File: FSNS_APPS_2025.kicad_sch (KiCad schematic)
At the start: 28 parts, among them J1 Conn_01x04_Pin, J2 Conn_01x03_Pin, J3 Conn_01x03_Pin, U1 STM32F103C8T6, U2 MCP6001-OT, U3 MCP6001-OT, Y1 16MHz

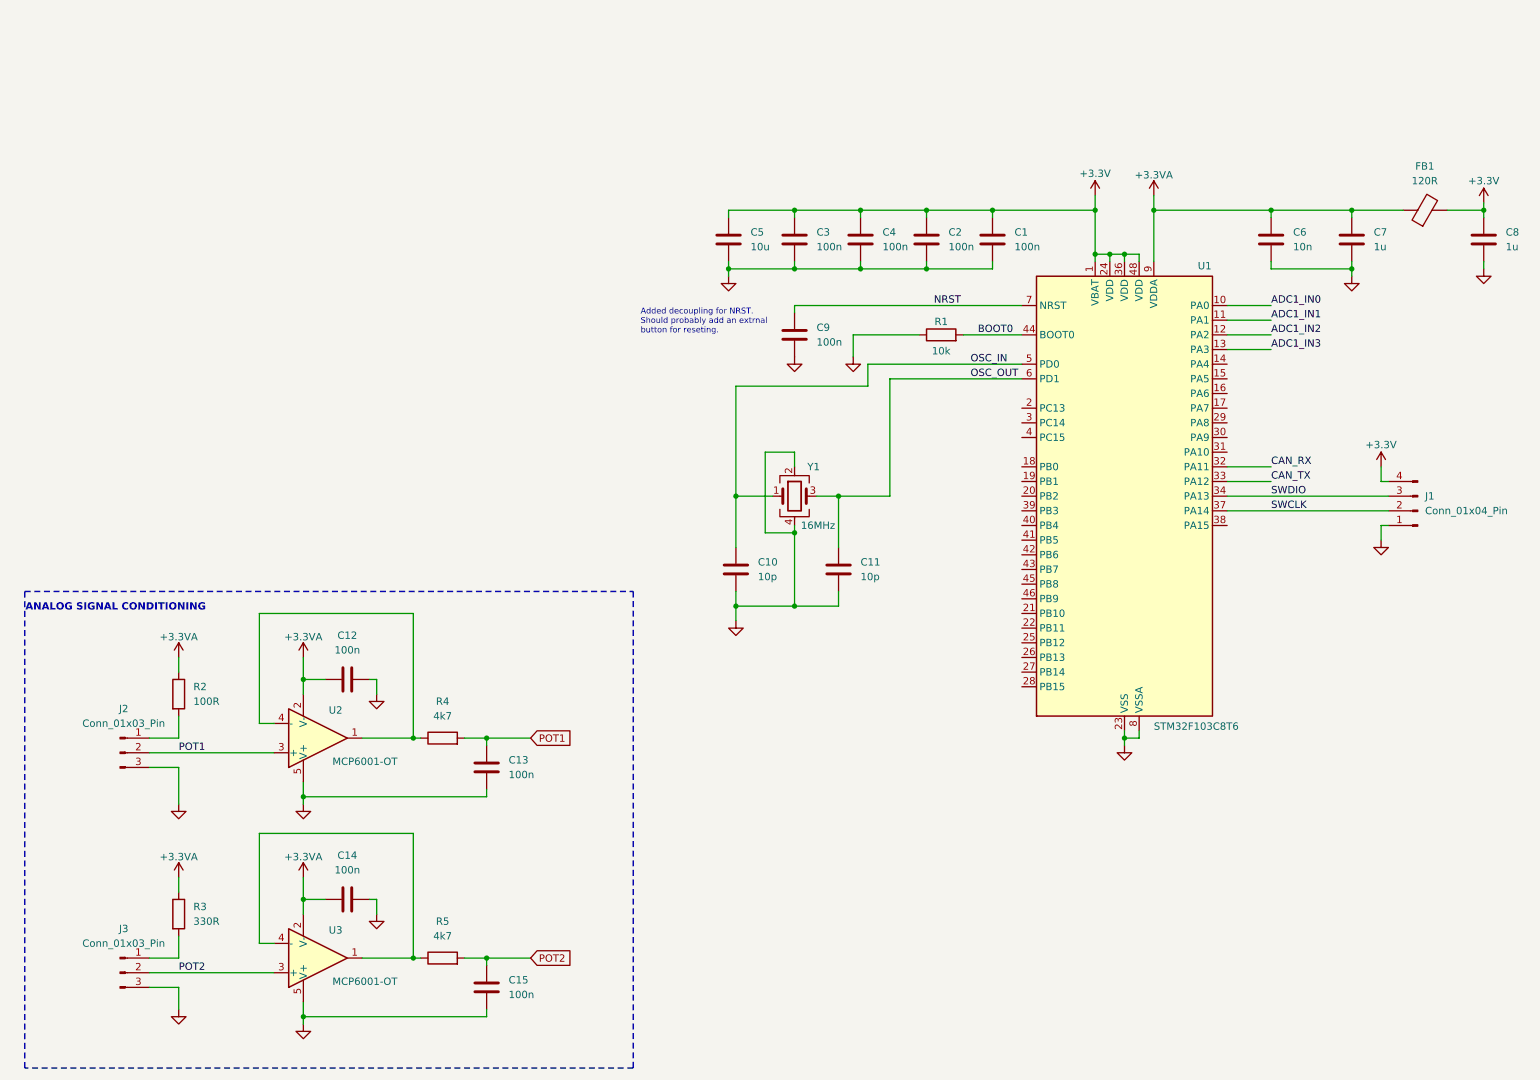
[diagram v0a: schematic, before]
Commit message: Added a few components.
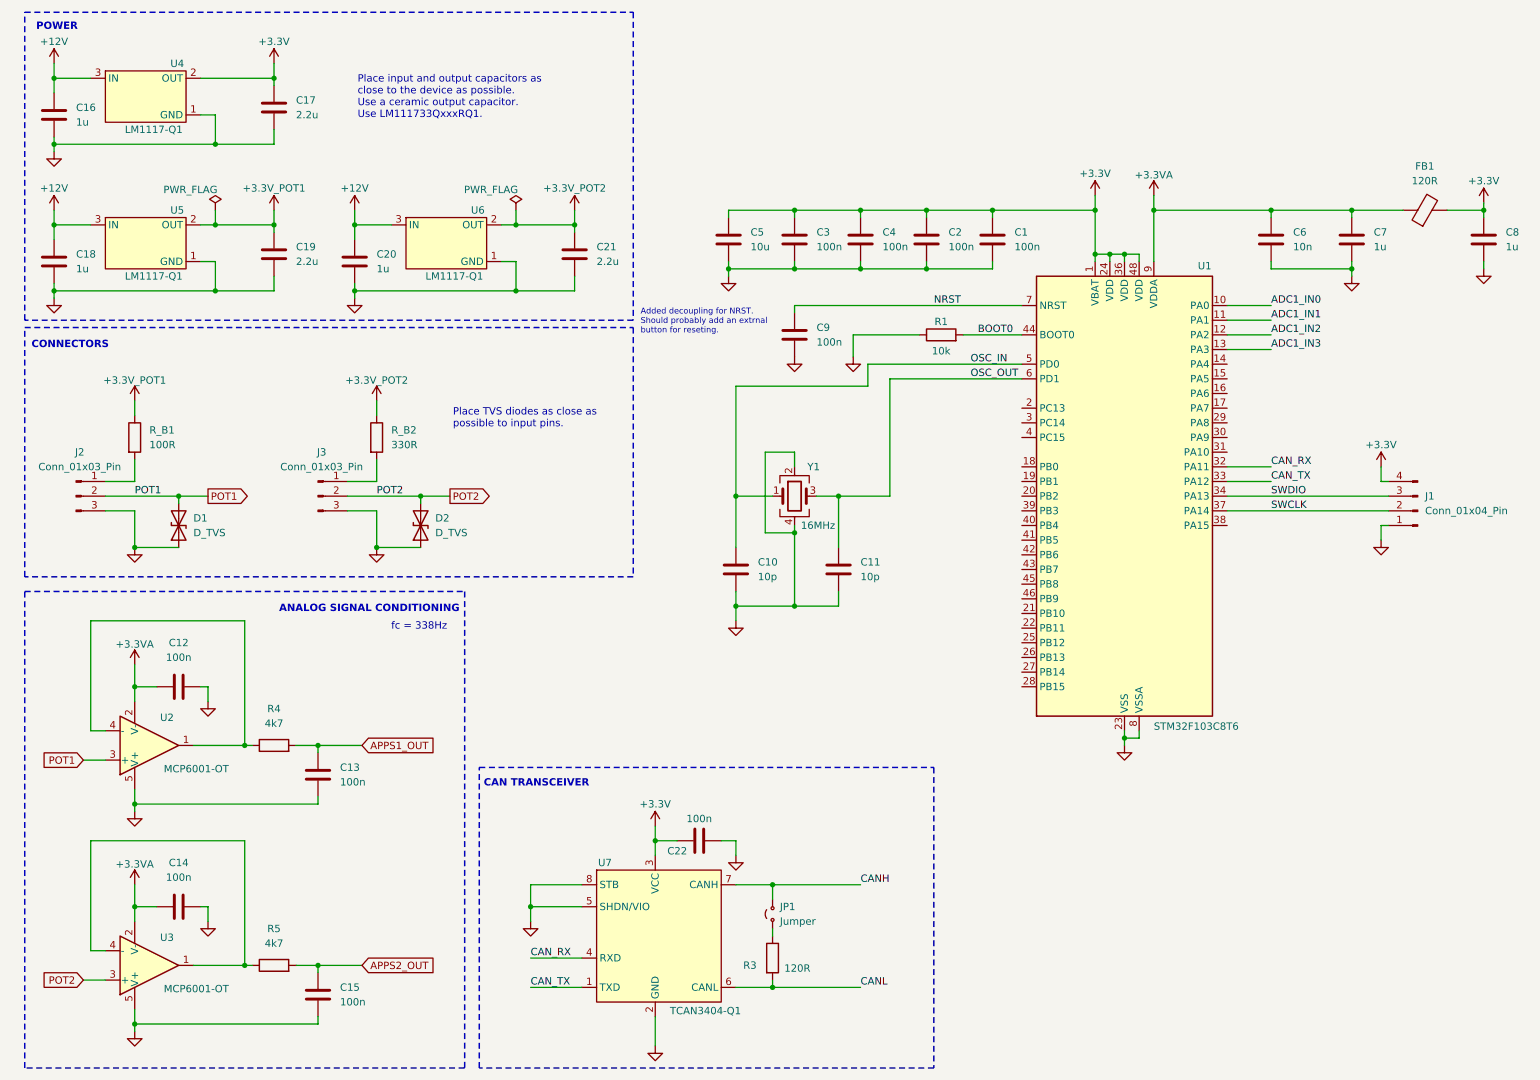
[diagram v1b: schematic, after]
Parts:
- added C16, C18, C20: 1u, symbol Device:C
- added C17, C19, C21: 2.2u, symbol Device:C
- added C22: 100n, symbol Device:C
- added D1, D2: D_TVS, symbol Device:D_TVS
- added JP1: Jumper, symbol Jumper:Jumper_2_Small_Open
- added R3: 120R, symbol Device:R
- added U4, U5, U6: LM1117-Q1, Package_TO_SOT_SMD:SOT-223-3_TabPin2, symbol TI_Linear_regulator:LM1117-Q1_18V_1A
- added U7: TCAN3404-Q1, Package_SO:SOIC-8-1EP_3.9x4.9mm_P1.27mm_EP2.95x4.9mm_Mask2.71x3.4mm, symbol TCAN340x:TCAN340x
- renumbered R2 to R_B1, R3 to R_B2
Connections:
- net +3.3V: now also C17.1, C22.1, U4.2 (OUT), U7.3 (VCC)
- net +3.3VA: no longer R_B1.1, R_B2.1
- net CAN_RX: now also U7.4 (RXD)
- net CAN_TX: now also U7.1 (TXD)
- net GND: now also C16.2, C17.2, C18.2, C19.2, C20.2, C21.2, C22.2, D1.1 (A1), D2.1 (A1), U4.1 (GND), U5.1 (GND), U6.1 (GND), U7.2 (GND), U7.5 (SHDN/VIO), U7.8 (STB)
- net POT1: now also D1.2 (A2); no longer C13.2, R4.2
- net POT2: now also D2.2 (A2); no longer C15.2, R5.2
- new net: JP1.1 (A), R3.1
- new net +12V: C16.1, C18.1, C20.1, U4.3 (IN), U5.3 (IN), U6.3 (IN)
- new net +3.3V_POT1: C19.1, R_B1.1, U5.2 (OUT)
- new net +3.3V_POT2: C21.1, R_B2.1, U6.2 (OUT)
- new net APPS1_OUT: C13.2, R4.2
- new net APPS2_OUT: C15.2, R5.2
- new net CANH: JP1.2 (B), U7.7 (CANH)
- new net CANL: R3.2, U7.6 (CANL)
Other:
- note added: "CAN TRANSCEIVER"
- note added: "CONNECTORS"
- note added: "POWER"
- note added: "Place TVS diodes as close as possible to input pins."
- note added: "Place input and output capacitors as close to the device as possible. Use a ceramic output capacitor. Use LM111733QxxxRQ1."
- note added: "fc = 338Hz"
- moved on the sheet: C12, C13, C14, C15, J2, J3, R4, R5, R_B1, R_B2, U2, U3
